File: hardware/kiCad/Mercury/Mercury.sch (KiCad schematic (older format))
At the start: 73 parts, among them J1 SWD, J10 OUTPUT, J11 Analog I/O, J12 Power Rails, J2 UART1, J3 I2C2, J4 UART1, J5 SPI1, J6 SPI2, J7 629105150521, J8 Battery Input, J9 INPUT, Q1 AO3401A, SW1 SW_SPDT, U1 STM32F407VGT6, U2 AMS1117-3.3, U3 AMS1117-5.0, Y1 HSE 16MHz

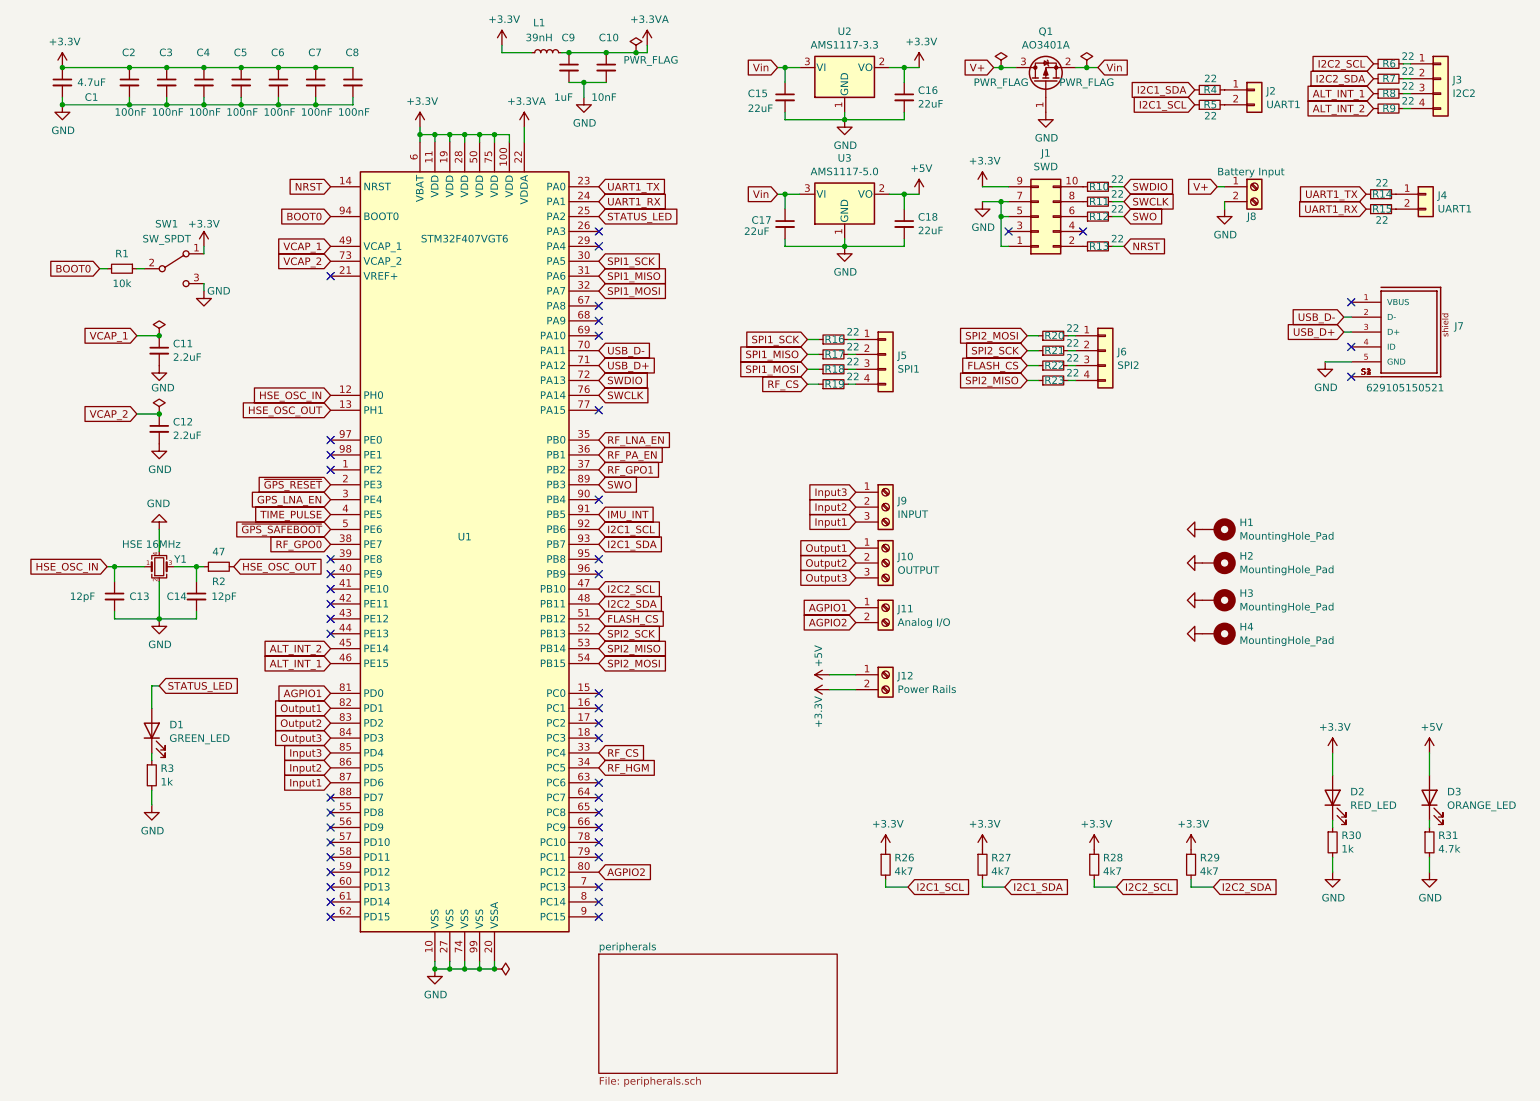
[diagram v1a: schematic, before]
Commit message: Layout Done
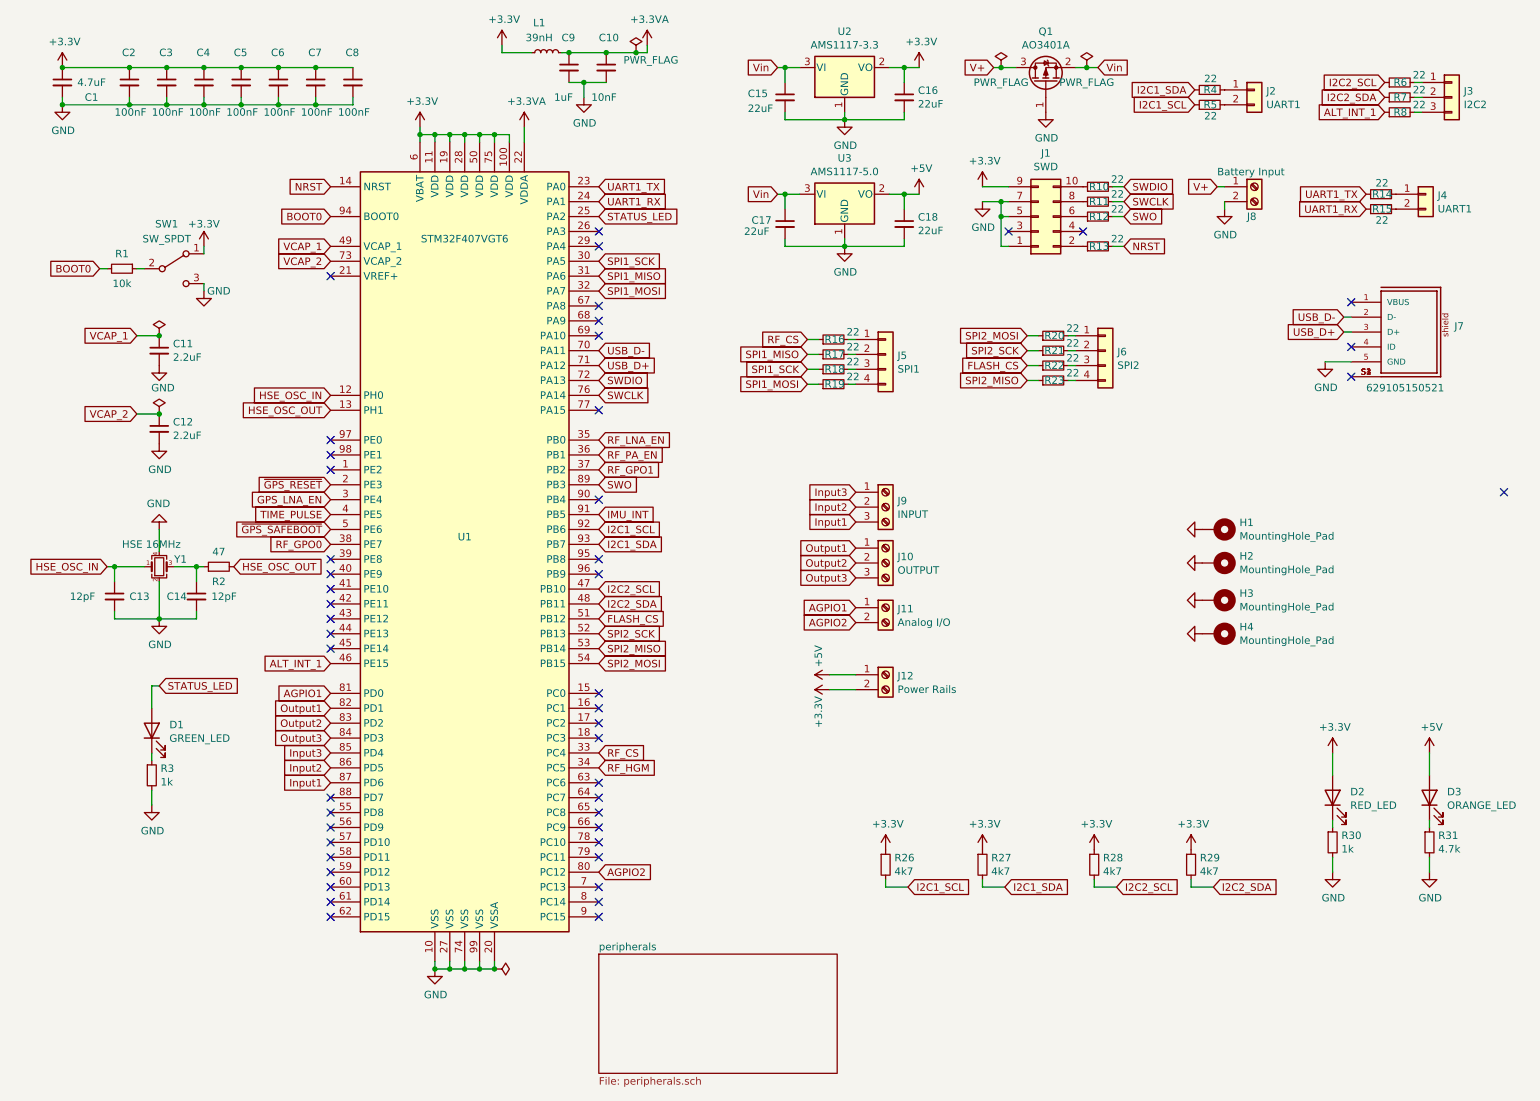
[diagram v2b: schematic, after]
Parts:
- removed J3: I2C2, Connector_Wire:SolderWire-0.1sqmm_1x04_P3.6mm_D0.4mm_OD1mm, symbol Connector_Generic:Conn_01x04
- removed R9: 22, Resistor_SMD:R_0402_1005Metric, symbol Device:R_Small
- added J3: I2C2, Connector_Wire:SolderWire-0.1sqmm_1x03_P3.6mm_D0.4mm_OD1mm, symbol Connector_Generic:Conn_01x03
- J8: footprint TerminalBlock_Phoenix:TerminalBlock_Phoenix_MKDS-3-2-5.08_1x02_P5.08mm_Horizontal -> TerminalBlock_Phoenix:TerminalBlock_Phoenix_MKDS-1,5-2-5.08_1x02_P5.08mm_Horizontal
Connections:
- net RF_CS: now also R16.1; no longer R19.1
- net SPI1_MOSI: now also R19.1; no longer R18.1
- net SPI1_SCK: now also R18.1; no longer R16.1
- net at R6.2: now also J3.1 (Pin_1)
- net at R7.2: now also J3.2 (Pin_2)
- net at R8.2: now also J3.3 (Pin_3)
- net ALT_INT_2: no longer names the net of U1.45 (PE14)
- no-connect marks 46 -> 48
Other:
- moved on the sheet: R6, R7, R8
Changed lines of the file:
@@
 F 0 "J8" H 8650 1600 50  0000 L CNN
 F 1 "Battery Input" H 8450 1900 50  0000 L CNN
-F 2 "TerminalBlock_Phoenix:TerminalBlock_Phoenix_MKDS-3-2-5.08_1x02_P5.08mm_Horizontal" H 8700 1800 50  0001 C CNN
+F 2 "TerminalBlock_Phoenix:TerminalBlock_Phoenix_MKDS-1,5-2-5.08_1x02_P5.08mm_Horizontal" H 8700 1800 50  0001 C CNN
 F 3 "~" H 8700 1800 50  0001 C CNN
 	1    8700 1800
@@
 Text GLabel 8300 1150 0    50   Input ~ 0
 I2C1_SDA
-Text GLabel 9500 975  0    50   Input ~ 0
+Text GLabel 9575 1100 0    50   Input ~ 0
 I2C2_SCL
 Text GLabel 9450 1850 0    50   Input ~ 0
@@
 L Device:R_Small R6
 U 1 1 5FEBD667
-P 9600 975
-F 0 "R6" V 9600 925 50  0000 L CNN
-F 1 "22" V 9650 800 50  0000 L CNN
-F 2 "Resistor_SMD:R_0402_1005Metric" H 9600 975 50  0001 C CNN
-F 3 "~" H 9600 975 50  0001 C CNN
-	1    9600 975
+P 9675 1100
+F 0 "R6" V 9675 1050 50  0000 L CNN
+F 1 "22" V 9725 925 50  0000 L CNN
+F 2 "Resistor_SMD:R_0402_1005Metric" H 9675 1100 50  0001 C CNN
+F 3 "~" H 9675 1100 50  0001 C CNN
+	1    9675 1100
 	0    -1   -1   0
 $EndComp
@@
 L Device:R_Small R7
 U 1 1 5FEBDD35
-P 9600 1075
-F 0 "R7" V 9600 1025 50  0000 L CNN
-F 1 "22" V 9650 900 50  0000 L CNN
-F 2 "Resistor_SMD:R_0402_1005Metric" H 9600 1075 50  0001 C CNN
-F 3 "~" H 9600 1075 50  0001 C CNN
-	1    9600 1075
+P 9675 1200
+F 0 "R7" V 9675 1150 50  0000 L CNN
+F 1 "22" V 9725 1025 50  0000 L CNN
+F 2 "Resistor_SMD:R_0402_1005Metric" H 9675 1200 50  0001 C CNN
+F 3 "~" H 9675 1200 50  0001 C CNN
+	1    9675 1200
 	0    -1   -1   0
 $EndComp
 Text GLabel 8425 6500 2    50   Input ~ 0
 I2C2_SDA
-Text GLabel 9500 1075 0    50   Input ~ 0
+Text GLabel 9575 1200 0    50   Input ~ 0
 I2C2_SDA
 $Comp
@@
 Text GLabel 4300 4700 2    50   Input ~ 0
 FLASH_CS
-Text GLabel 2500 4900 0    50   Input ~ 0
-ALT_INT_2
 Text GLabel 2500 5000 0    50   Input ~ 0
 ALT_INT_1
@@
 RF_GPO0
 Wire Wire Line
-	9700 1075 9750 1075
-Wire Wire Line
-	9700 975  9750 975
+	9775 1200 9825 1200
+Wire Wire Line
+	9775 1100 9825 1100
 $Comp
 L Device:R_Small R8
 U 1 1 5FECDB5E
-P 9600 1175
-F 0 "R8" V 9600 1125 50  0000 L CNN
-F 1 "22" V 9650 1000 50  0000 L CNN
-F 2 "Resistor_SMD:R_0402_1005Metric" H 9600 1175 50  0001 C CNN
-F 3 "~" H 9600 1175 50  0001 C CNN
-	1    9600 1175
-	0    -1   -1   0
-$EndComp
-$Comp
-L Device:R_Small R9
-U 1 1 5FECDB68
-P 9600 1275
-F 0 "R9" V 9600 1225 50  0000 L CNN
-F 1 "22" V 9650 1100 50  0000 L CNN
-F 2 "Resistor_SMD:R_0402_1005Metric" H 9600 1275 50  0001 C CNN
-F 3 "~" H 9600 1275 50  0001 C CNN
-	1    9600 1275
-	0    -1   -1   0
-$EndComp
-Wire Wire Line
-	9700 1275 9750 1275
-Wire Wire Line
-	9700 1175 9750 1175
-Text GLabel 9500 1275 0    50   Input ~ 0
-ALT_INT_2
-Text GLabel 9500 1175 0    50   Input ~ 0
+P 9675 1300
+F 0 "R8" V 9675 1250 50  0000 L CNN
+F 1 "22" V 9725 1125 50  0000 L CNN
+F 2 "Resistor_SMD:R_0402_1005Metric" H 9675 1300 50  0001 C CNN
+F 3 "~" H 9675 1300 50  0001 C CNN
+	1    9675 1300
+	0    -1   -1   0
+$EndComp
+Wire Wire Line
+	9775 1300 9825 1300
+Text GLabel 9575 1300 0    50   Input ~ 0
 ALT_INT_1
 $Comp
@@
 Wire Wire Line
 	5975 3025 6025 3025
-Text GLabel 5700 2825 0    50   Input ~ 0
+Text GLabel 5700 3025 0    50   Input ~ 0
 SPI1_SCK
 Wire Wire Line
@@
 Wire Wire Line
 	5700 2925 5775 2925
-Text GLabel 5700 3025 0    50   Input ~ 0
+Text GLabel 5700 3125 0    50   Input ~ 0
 SPI1_MOSI
 Wire Wire Line
 	5700 3025 5775 3025
-Text GLabel 5700 3125 0    50   Input ~ 0
+Text GLabel 5700 2825 0    50   Input ~ 0
 RF_CS
 Wire Wire Line
@@
 	1    0    0    -1
 $EndComp
-$Comp
-L Connector_Generic:Conn_01x04 J3
-U 1 1 60266721
-P 9950 1075
-F 0 "J3" H 10030 1067 50  0000 L CNN
-F 1 "I2C2" H 10030 976 50  0000 L CNN
-F 2 "Connector_Wire:SolderWire-0.1sqmm_1x04_P3.6mm_D0.4mm_OD1mm" H 9950 1075 50  0001 C CNN
-F 3 "~" H 9950 1075 50  0001 C CNN
-	1    9950 1075
-	1    0    0    -1
-$EndComp
 NoConn ~ 4300 6000
 NoConn ~ 4300 6100
 NoConn ~ 4300 2600
+NoConn ~ 2500 4900
+NoConn ~ 10375 3850
+$Comp
+L Connector_Generic:Conn_01x03 J3
+U 1 1 600074F1
+P 10025 1200
+F 0 "J3" H 10105 1242 50  0000 L CNN
+F 1 "I2C2" H 10105 1151 50  0000 L CNN
+F 2 "Connector_Wire:SolderWire-0.1sqmm_1x03_P3.6mm_D0.4mm_OD1mm" H 10025 1200 50  0001 C CNN
+F 3 "~" H 10025 1200 50  0001 C CNN
+	1    10025 1200
+	1    0    0    -1
+$EndComp
 $EndSCHEMATC
